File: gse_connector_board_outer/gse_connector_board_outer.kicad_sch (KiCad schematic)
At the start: 8 parts, among them J1 arming_connector, J2 gse_com_connector, J3 chg_connector, J5 Conn_02x02_Top_Bottom, J7 Conn_02x02_Top_Bottom, J8 Conn_02x02_Top_Bottom

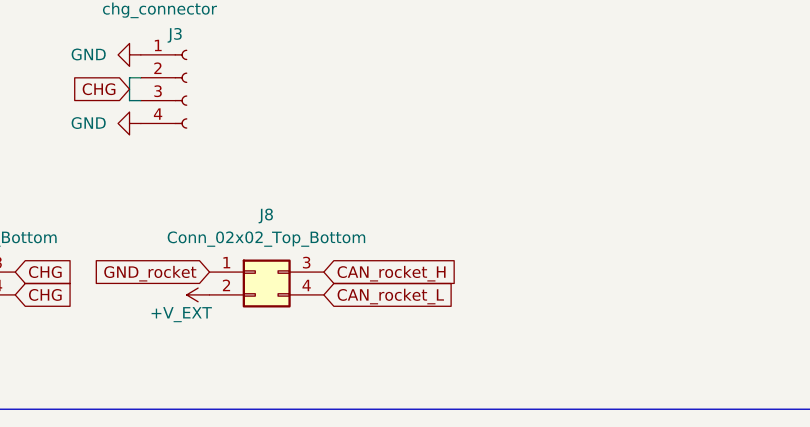
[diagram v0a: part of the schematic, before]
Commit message: final touches
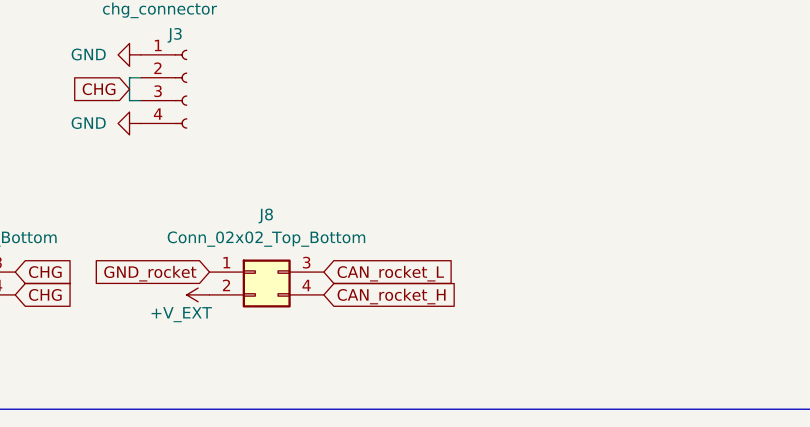
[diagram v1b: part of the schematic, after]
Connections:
- net CAN_rocket_H: now also J8.4 (Pin_4); no longer J8.3 (Pin_3)
- net CAN_rocket_L: now also J8.3 (Pin_3); no longer J8.4 (Pin_4)
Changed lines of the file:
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@@
+		)
+	)
+	(text "GSE interface (no CAN isolation; termination is switched on the inner board)\nJ8 connects straight through to the magnetic J2. GND_rocket is the common CAN ground\n(tied to GND on the inner board). Terminate the GSE end of the bus with 120 Ohm.\n+V_EXT (J8.2 -> J2.1): supplied by the GSE whenever it is connected (12 V assumed, ~5 mA).\nIt opens the rocket-side termination; without it the bus has three terminations."
+		(exclude_from_sim no)
+		(at 96.52 50.8 0)
+		(effects
+			(font
+				(size 1.27 1.27)
+			)
+			(justify left top)
 		)
 	)
@@
 	(wire
 		(pts
-			(xy 242.57 34.29) (xy 247.65 34.29)
+			(xy 118.11 80.01) (xy 104.14 80.01)
 		)
 		(stroke
@@
 		)
 	)
+	(wire
+		(pts
+			(xy 242.57 34.29) (xy 247.65 34.29)
+		)
+		(stroke
+			(width 0)
+			(type default)
+		)
+	)
 	(global_label "CAN_rocket_H"
 		(shape input)
@@
 	(global_label "CAN_rocket_H"
 		(shape input)
-		(at 196.85 104.14 0)
+		(at 196.85 106.68 0)
 		(fields_autoplaced yes)
 		(effects
@@
 		)
 		(property "Intersheetrefs" "${INTERSHEET_REFS}"
-			(at 209.4509 104.14 0)
+			(at 209.4509 106.68 0)
 			(hide yes)
 			(show_name no)
@@
 		)
 	)
+	(global_label "GND_rocket"
+		(shape input)
+		(at 184.15 104.14 180)
+		(fields_autoplaced yes)
+		(effects
+			(font
+				(size 1.27 1.27)
+			)
+			(justify right)
+		)
+		(property "Intersheetrefs" "${INTERSHEET_REFS}"
+			(at 174.244 104.14 0)
+			(hide yes)
+			(show_name no)
+			(do_not_autoplace no)
+			(effects
+				(font
+					(size 1.27 1.27)
+				)
+				(justify right)
+			)
+		)
+	)
 	(global_label "CHG"
 		(shape input)
@@
 	(global_label "CAN_rocket_L"
 		(shape input)
-		(at 196.85 106.68 0)
+		(at 196.85 104.14 0)
 		(fields_autoplaced yes)
 		(effects
@@
 		)
 		(property "Intersheetrefs" "${INTERSHEET_REFS}"
-			(at 209.1485 106.68 0)
+			(at 209.1485 104.14 0)
 			(hide yes)
 			(show_name no)
@@
 	)
 	(symbol
+		(lib_id "power:VCC")
+		(at 104.14 80.01 0)
+		(unit 1)
+		(body_style 1)
+		(exclude_from_sim no)
+		(in_bom yes)
+		(on_board yes)
+		(in_pos_files yes)
+		(dnp no)
+		(property "Reference" "#PWR072"
+			(at 104.14 83.82 0)
+			(hide yes)
+			(show_name no)
+			(do_not_autoplace no)
+			(effects
+				(font
+					(size 1.27 1.27)
+				)
+			)
+		)
+		(property "Value" "+V_EXT"
+			(at 104.14 76.2 0)
+			(show_name no)
+			(do_not_autoplace no)
+			(effects
+				(font
+					(size 1.27 1.27)
+				)
+			)
+		)
+		(property "Footprint" ""
+			(at 104.14 80.01 0)
+			(hide yes)
+			(show_name no)
+			(do_not_autoplace no)
+			(effects
+				(font
+					(size 1.27 1.27)
+				)
+			)
+		)
+		(property "Datasheet" ""
+			(at 104.14 80.01 0)
+			(hide yes)
+			(show_name no)
+			(do_not_autoplace no)
+			(effects
+				(font
+					(size 1.27 1.27)
+				)
+			)
+		)
+		(property "Description" "Power symbol creates a global label with name \"VCC\""
+			(at 104.14 80.01 0)
+			(hide yes)
+			(show_name no)
+			(do_not_autoplace no)
+			(effects
+				(font
+					(size 1.27 1.27)
+				)
+			)
+		)
+		(pin "1"
+		)
+		(instances
+			(project "gse_connector_board_outer"
+				(path "/df677c4e-51be-471c-a547-b22db5b9f5a1"
+					(reference "#PWR072")
+					(unit 1)
+				)
+			)
+		)
+	)
+	(symbol
 		(lib_name "GND_1")
 		(lib_id "power:GND")
@@
 		)
 	)
-	(global_label "GND_rocket"
-		(shape input)
-		(at 184.15 104.14 180)
-		(fields_autoplaced yes)
-		(effects
-			(font
-				(size 1.27 1.27)
-			)
-			(justify right)
-		)
-		(property "Intersheetrefs" "${INTERSHEET_REFS}"
-			(at 174.2440 104.14 0)
-			(hide yes)
-			(show_name no)
-			(do_not_autoplace no)
-			(effects
-				(font
-					(size 1.27 1.27)
-				)
-				(justify right)
-			)
-		)
-	)
-	(symbol
-		(lib_id "power:VCC")
-		(at 104.14 80.01 0)
-		(unit 1)
-		(body_style 1)
-		(exclude_from_sim no)
-		(in_bom yes)
-		(on_board yes)
-		(in_pos_files yes)
-		(dnp no)
-		(property "Reference" "#PWR072"
-			(at 104.14 83.82 0)
-			(hide yes)
-			(show_name no)
-			(do_not_autoplace no)
-			(effects
-				(font
-					(size 1.27 1.27)
-				)
-			)
-		)
-		(property "Value" "+V_EXT"
-			(at 104.14 76.2 0)
-			(show_name no)
-			(do_not_autoplace no)
-			(effects
-				(font
-					(size 1.27 1.27)
-				)
-			)
-		)
-		(property "Footprint" ""
-			(at 104.14 80.01 0)
-			(hide yes)
-			(show_name no)
-			(do_not_autoplace no)
-			(effects
-				(font
-					(size 1.27 1.27)
-				)
-			)
-		)
-		(property "Datasheet" ""
-			(at 104.14 80.01 0)
-			(hide yes)
-			(show_name no)
-			(do_not_autoplace no)
-			(effects
-				(font
-					(size 1.27 1.27)
-				)
-			)
-		)
-		(property "Description" "Power symbol creates a global label with name \"VCC\""
-			(at 104.14 80.01 0)
-			(hide yes)
-			(show_name no)
-			(do_not_autoplace no)
-			(effects
-				(font
-					(size 1.27 1.27)
-				)
-			)
-		)
-		(pin "1"
-		)
-		(instances
-			(project "gse_connector_board_outer"
-				(path "/df677c4e-51be-471c-a547-b22db5b9f5a1"
-					(reference "#PWR072")
-					(unit 1)
-				)
-			)
-		)
-	)
-	(text "GSE interface (no CAN isolation; termination is switched on the inner board)\nJ8 connects straight through to the magnetic J2. GND_rocket is the common CAN ground\n(tied to GND on the inner board). Terminate the GSE end of the bus with 120 Ohm.\n+V_EXT (J8.2 -> J2.1): supplied by the GSE whenever it is connected (12 V assumed, ~5 mA).\nIt opens the rocket-side termination; without it the bus has three terminations."
-		(exclude_from_sim no)
-		(at 96.52 50.8 0)
-		(effects
-			(font
-				(size 1.27 1.27)
-			)
-			(justify left top)
-		)
-	)
-	(wire
-		(pts
-			(xy 118.11 80.01) (xy 104.14 80.01)
-		)
-		(stroke
-			(width 0)
-			(type default)
-		)
-	)

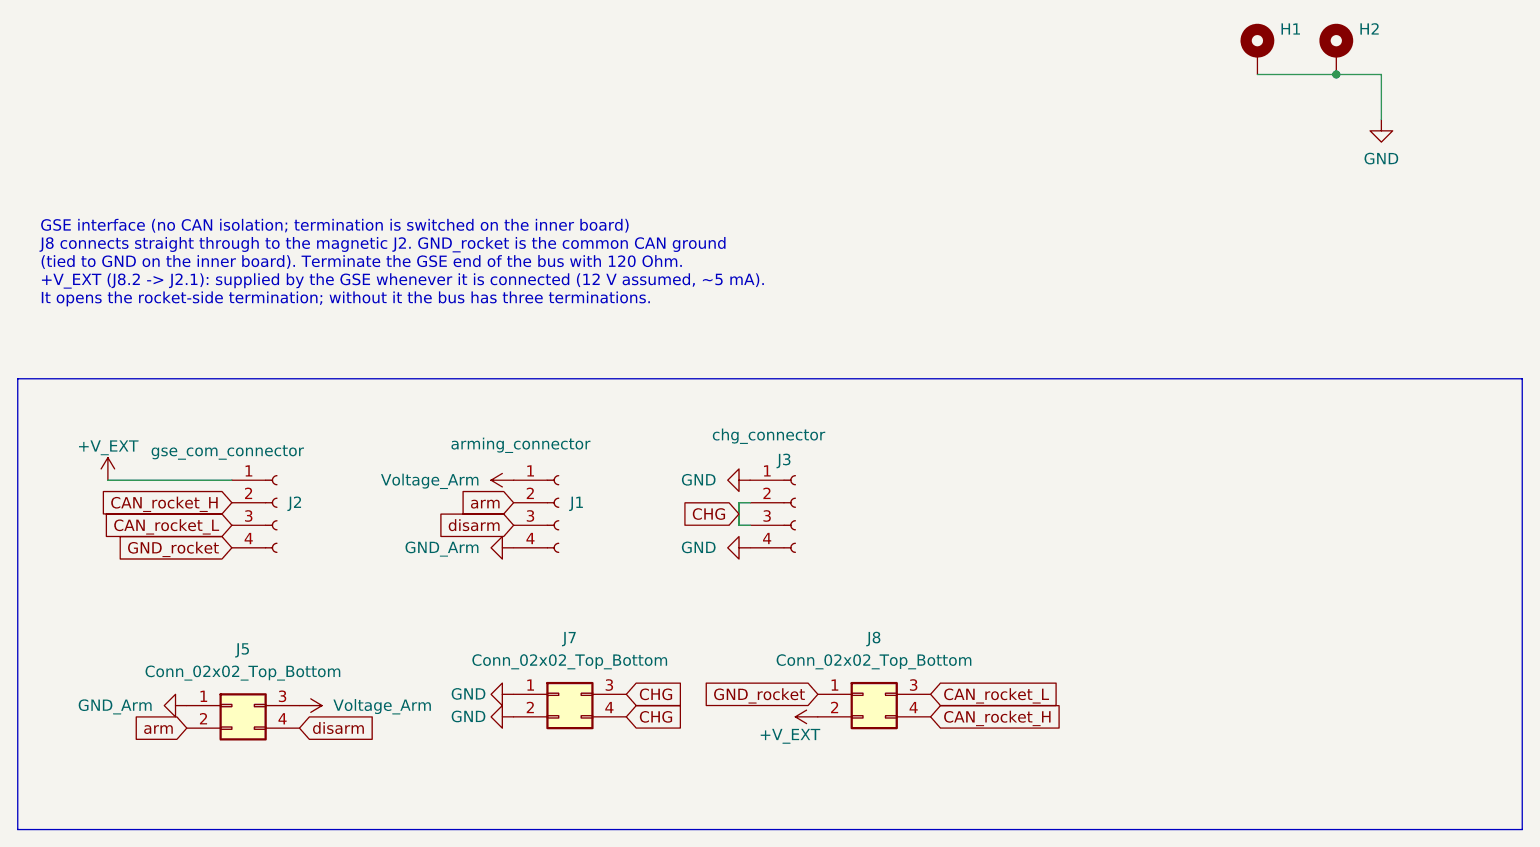
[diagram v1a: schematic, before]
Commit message: final ordered version
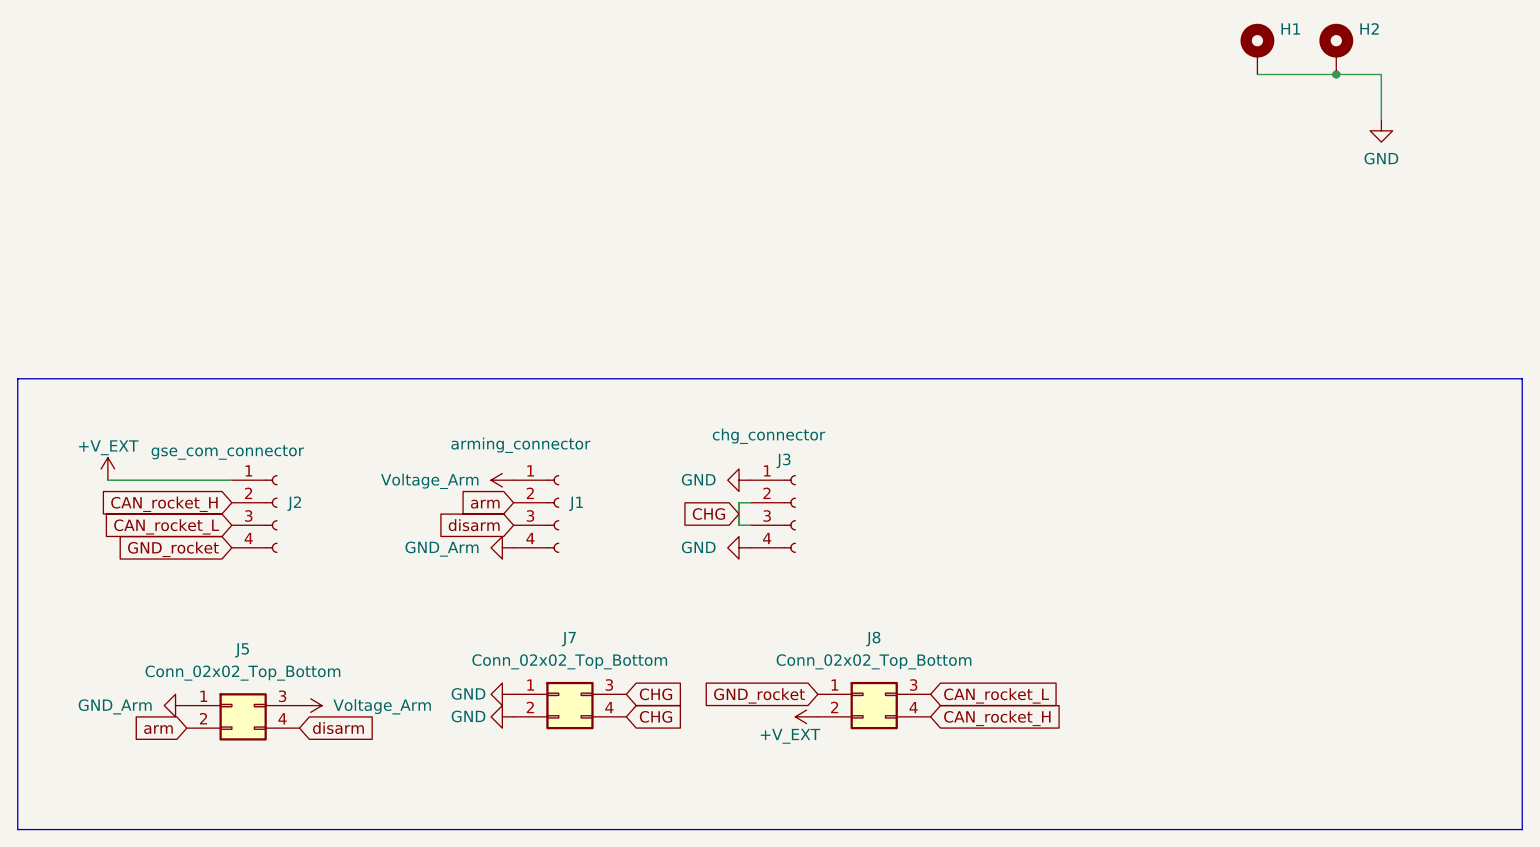
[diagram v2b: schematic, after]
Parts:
- J1, J2, J3: footprint custom_parts:4_pin_mag_con_mv_adapt -> custom_parts:4_pin_mag_con_flat_mv_adapt
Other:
- note removed: "GSE interface (no CAN isolation; termination is switched on the inner board) J8 connects straight through to the magnetic J2. GND_rocket is the common CAN ground (tied to GND on the inner board). Terminate the GSE end of the bus with 120 Ohm. +V_EXT (J8.2 -> J2.1): supplied by the GSE whenever it is connected (12 V assumed, ~5 mA). It opens the rocket-side termination; without it the bus has thre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"
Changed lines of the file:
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@@
-		)
-	)
-	(text "GSE interface (no CAN isolation; termination is switched on the inner board)\nJ8 connects straight through to the magnetic J2. GND_rocket is the common CAN ground\n(tied to GND on the inner board). Terminate the GSE end of the bus with 120 Ohm.\n+V_EXT (J8.2 -> J2.1): supplied by the GSE whenever it is connected (12 V assumed, ~5 mA).\nIt opens the rocket-side termination; without it the bus has three terminations."
-		(exclude_from_sim no)
-		(at 96.52 50.8 0)
-		(effects
-			(font
-				(size 1.27 1.27)
-			)
-			(justify left top)
 		)
 	)
@@
 			)
 		)
-		(property "Footprint" "custom_parts:4_pin_mag_con_mv_adapt"
+		(property "Footprint" "custom_parts:4_pin_mag_con_flat_mv_adapt"
 			(at 181.61 82.55 0)
 			(hide yes)
@@
 			)
 		)
-		(property "Footprint" "custom_parts:4_pin_mag_con_mv_adapt"
+		(property "Footprint" "custom_parts:4_pin_mag_con_flat_mv_adapt"
 			(at 154.94 82.55 0)
 			(hide yes)
@@
 			)
 		)
-		(property "Footprint" "custom_parts:4_pin_mag_con_mv_adapt"
+		(property "Footprint" "custom_parts:4_pin_mag_con_flat_mv_adapt"
 			(at 123.19 82.55 0)
 			(hide yes)
